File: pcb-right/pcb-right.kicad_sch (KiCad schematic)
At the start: 91 parts, among them J1 Conn_01x02_Pin, J2 Conn_01x06_MountingPin, J3 Conn_01x04_Pin, SW1 SW_Push, SW2 Rotary_Encoder_Default, U1 XC6206PxxxMR, U2 STM32F401RCTx, Y1 12MHz

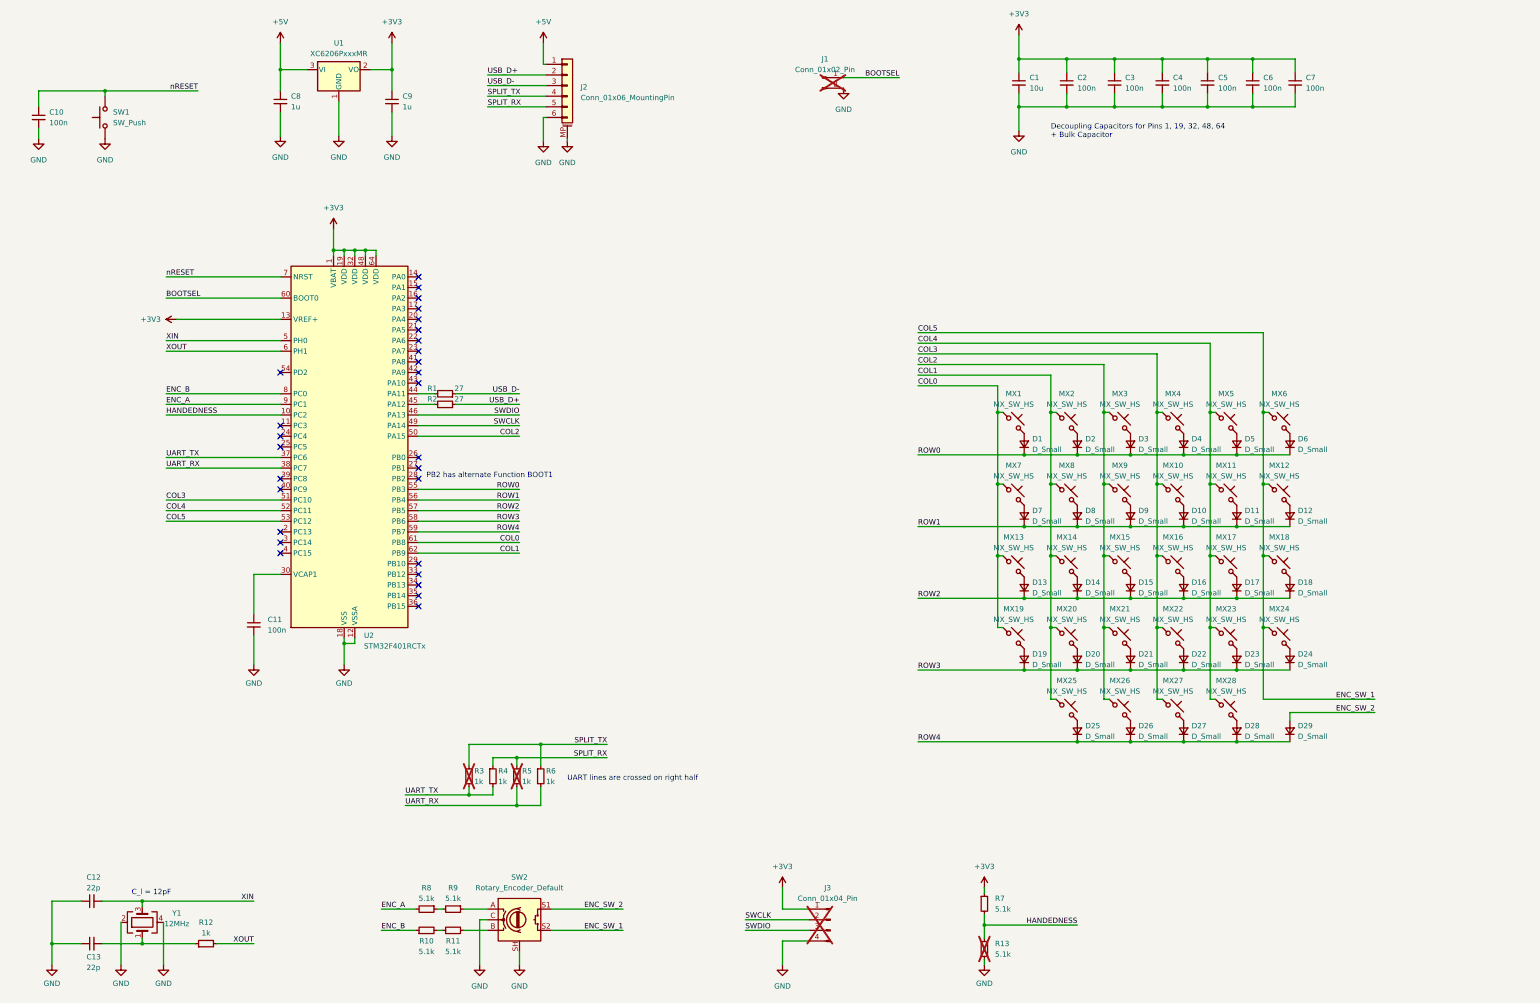
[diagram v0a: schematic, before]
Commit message: quick save
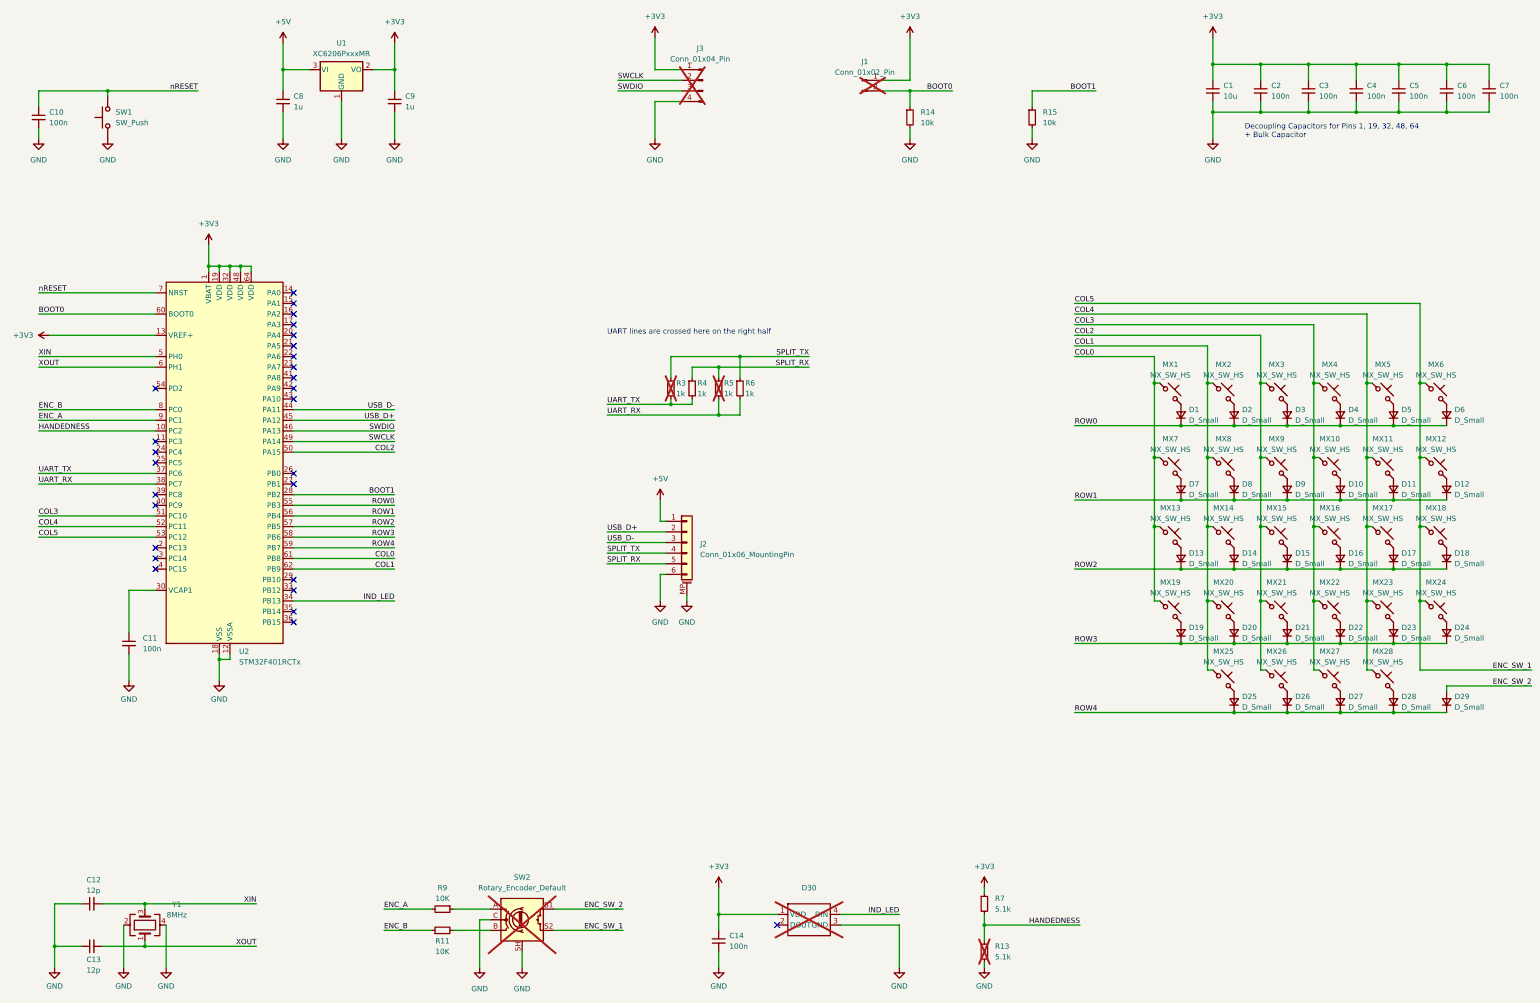
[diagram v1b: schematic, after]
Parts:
- removed R1, R2: 27, Resistor_SMD:R_0603_1608Metric_Pad0.98x0.95mm_HandSolder, symbol Device:R_Small
- removed R10, R8: 5.1k, Resistor_SMD:R_0603_1608Metric_Pad0.98x0.95mm_HandSolder, symbol Device:R_Small
- removed R12: 1k, Resistor_SMD:R_0603_1608Metric_Pad0.98x0.95mm_HandSolder, symbol Device:R_Small
- added C14: 100n, Capacitor_SMD:C_0603_1608Metric, symbol Device:C_Small
- added D30: ~, lib-zegonix:SK6812MINI-E_3.2x2.8_reverse_mount, symbol lib-zegonix:sk6812mini-e
- added R14, R15: 10k, Resistor_SMD:R_0603_1608Metric, symbol Device:R_Small
- C12, C13: value 22p -> 12p
- J2: footprint Connector_JST:JST_SHL_SM06B-SHLS-TF_1x06-1MP_P1.00mm_Horizontal -> Connector_JST:JST_SH_SM06B-SRSS-TB_1x06-1MP_P1.00mm_Horizontal
- R11, R9: value 5.1k -> 10K
- SW2: now not fitted; now left out of the parts list
- Y1: value 12MHz -> 8MHz
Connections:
- net +3V3: now also J1.1 (Pin_1), C14.1, D30.1 (VDD)
- net ENC_A: now also R9.2
- net ENC_B: now also R11.1
- net GND: now also C14.2, D30.3 (GND), R14.2, R15.2; no longer J1.2 (Pin_2)
- net USB_D+: now also U2.45 (PA12)
- net USB_D-: now also U2.44 (PA11)
- net XOUT: now also C13.2, Y1.1
- net BOOT1: now reaches U2.28 (PB2)
- net BOOT1: now also R15.1
- net IND_LED: now reaches U2.34 (PB13)
- net IND_LED: now also D30.4 (DIN)
- net BOOTSEL renamed BOOT0
- net BOOT0: now also J1.2 (Pin_2), R14.1; no longer J1.1 (Pin_1)
- no-connect marks 28 -> 27
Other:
- note added: "UART lines are crossed here on the right half"
- note removed: "C_l = 12pF"
- note removed: "PB2 has alternate Function BOOT1"
- note removed: "UART lines are crossed on right half"
- moved on the sheet: C1, C11, C12, C13, C2, C3, C4, C5, C6, C7, C8, C9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
